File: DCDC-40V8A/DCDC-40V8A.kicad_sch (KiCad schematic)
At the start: 2 parts, among them J3 Conn_01x09, J4 Conn_01x09

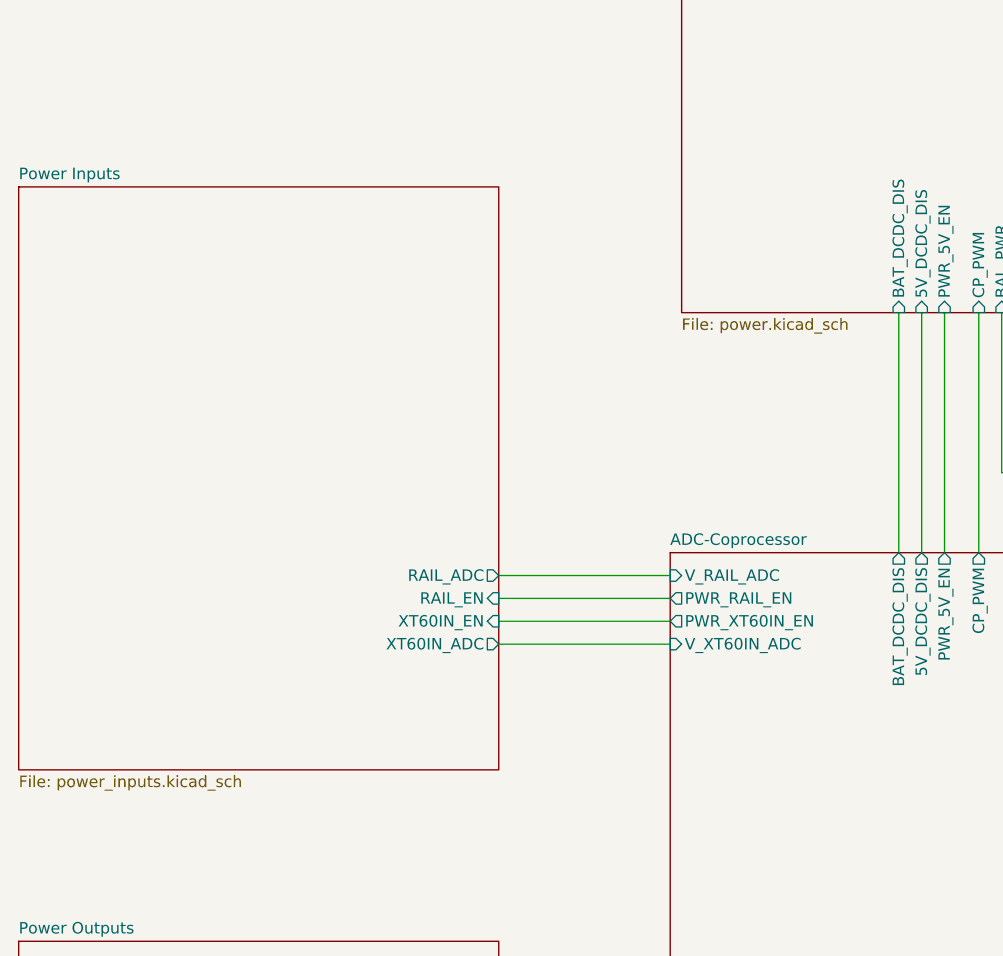
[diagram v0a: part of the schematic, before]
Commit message: wip before CP deletion
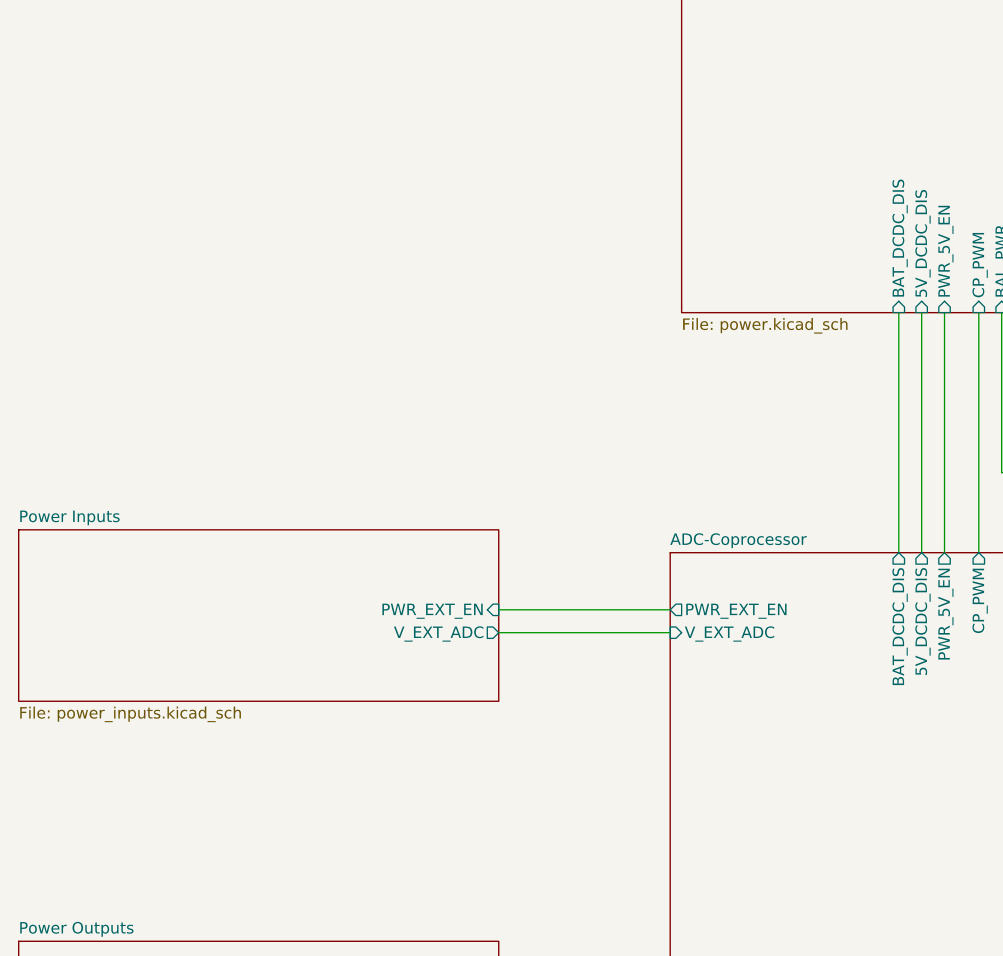
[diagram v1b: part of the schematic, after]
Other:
- sheet ADC-Coprocessor ports: added PWR_EXT_EN, V_EXT_ADC; removed PWR_RAIL_EN, PWR_XT60IN_EN, V_RAIL_ADC, V_XT60IN_ADC
- sheet Power Inputs ports: added PWR_EXT_EN, V_EXT_ADC; removed RAIL_ADC, RAIL_EN, XT60IN_ADC, XT60IN_EN
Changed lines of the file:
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@@
 	(wire
 		(pts
-			(xy 86.36 124.46) (xy 105.41 124.46)
+			(xy 86.36 128.27) (xy 105.41 128.27)
 		)
 		(stroke
@@
 	(wire
 		(pts
-			(xy 86.36 127) (xy 105.41 127)
-		)
-		(stroke
-			(width 0)
-			(type default)
-		)
-	)
-	(wire
-		(pts
 			(xy 309.88 110.49) (xy 309.88 171.45)
 		)
@@
 	(wire
 		(pts
-			(xy 86.36 129.54) (xy 105.41 129.54)
-		)
-		(stroke
-			(width 0)
-			(type default)
-		)
-	)
-	(wire
-		(pts
 			(xy 154.94 222.25) (xy 154.94 233.68)
 		)
@@
 	(wire
 		(pts
-			(xy 86.36 121.92) (xy 105.41 121.92)
+			(xy 86.36 125.73) (xy 105.41 125.73)
 		)
 		(stroke
@@
 			)
 		)
-		(pin "PWR_RAIL_EN" output
-			(at 105.41 124.46 180)
-			(effects
-				(font
-					(size 1.27 1.27)
-				)
-				(justify left)
-			)
-		)
-		(pin "PWR_XT60IN_EN" output
-			(at 105.41 127 180)
-			(effects
-				(font
-					(size 1.27 1.27)
-				)
-				(justify left)
-			)
-		)
-		(pin "V_RAIL_ADC" input
-			(at 105.41 121.92 180)
-			(effects
-				(font
-					(size 1.27 1.27)
-				)
-				(justify left)
-			)
-		)
-		(pin "V_XT60IN_ADC" input
-			(at 105.41 129.54 180)
+		(pin "PWR_EXT_EN" output
+			(at 105.41 125.73 180)
+			(effects
+				(font
+					(size 1.27 1.27)
+				)
+				(justify left)
+			)
+		)
+		(pin "V_EXT_ADC" input
+			(at 105.41 128.27 180)
 			(effects
 				(font
@@
 	)
 	(sheet
-		(at 33.02 78.74)
-		(size 53.34 64.77)
+		(at 33.02 116.84)
+		(size 53.34 19.05)
 		(exclude_from_sim no)
 		(in_bom yes)
@@
 		)
 		(property "Sheetname" "Power Inputs"
-			(at 33.02 78.0284 0)
+			(at 33.02 116.1284 0)
 			(show_name no)
 			(do_not_autoplace no)
@@
 		)
 		(property "Sheetfile" "power_inputs.kicad_sch"
-			(at 33.02 144.0946 0)
+			(at 33.02 136.4746 0)
 			(show_name no)
 			(do_not_autoplace no)
@@
 			)
 		)
-		(pin "RAIL_ADC" output
-			(at 86.36 121.92 0)
-			(effects
-				(font
-					(size 1.27 1.27)
-				)
-				(justify right)
-			)
-		)
-		(pin "RAIL_EN" input
-			(at 86.36 124.46 0)
-			(effects
-				(font
-					(size 1.27 1.27)
-				)
-				(justify right)
-			)
-		)
-		(pin "XT60IN_ADC" output
-			(at 86.36 129.54 0)
-			(effects
-				(font
-					(size 1.27 1.27)
-				)
-				(justify right)
-			)
-		)
-		(pin "XT60IN_EN" input
-			(at 86.36 127 0)
-			(effects
-				(font
+		(pin "V_EXT_ADC" output
+			(at 86.36 128.27 0)
+			(effects
+				(font
+					(size 1.27 1.27)
+				)
+				(justify right)
+			)
+		)
+		(pin "PWR_EXT_EN" input
+			(at 86.36 125.73 0)
+			(effects
+				(font
